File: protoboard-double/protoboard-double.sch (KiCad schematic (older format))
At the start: 23 parts, among them J1 MODULE_HEADER, J2 MODULE_HEADER, P1 CONN_01X22, P10 CONN_01X22, P11 CONN_01X22, P12 CONN_01X22, P13 CONN_01X22, P14 CONN_01X22, P15 CONN_01X22, P16 CONN_01X22, P17 CONN_01X22, P18 CONN_01X22, P19 CONN_01X22, P2 CONN_01X22, P3 CONN_01X22, P4 CONN_01X22, P5 CONN_01X22, P6 CONN_01X22, P7 CONN_01X22, P8 CONN_01X22, P9 CONN_01X22

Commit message: doublewide ready for production
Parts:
- SILK1: footprint parts:TESSEL-HEXAGON-LOGO -> parts:TESSEL-HEXAGON-LOGO-BACK
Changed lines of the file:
@@
 F 0 "SILK1" H 4750 1950 60  0000 C CNN
 F 1 "logo" H 4750 1850 60  0000 C CNN
-F 2 "parts:TESSEL-HEXAGON-LOGO" H 4750 1900 60  0001 C CNN
+F 2 "parts:TESSEL-HEXAGON-LOGO-BACK" H 4750 1900 60  0001 C CNN
 F 3 "" H 4750 1900 60  0000 C CNN
 	1    4750 1900

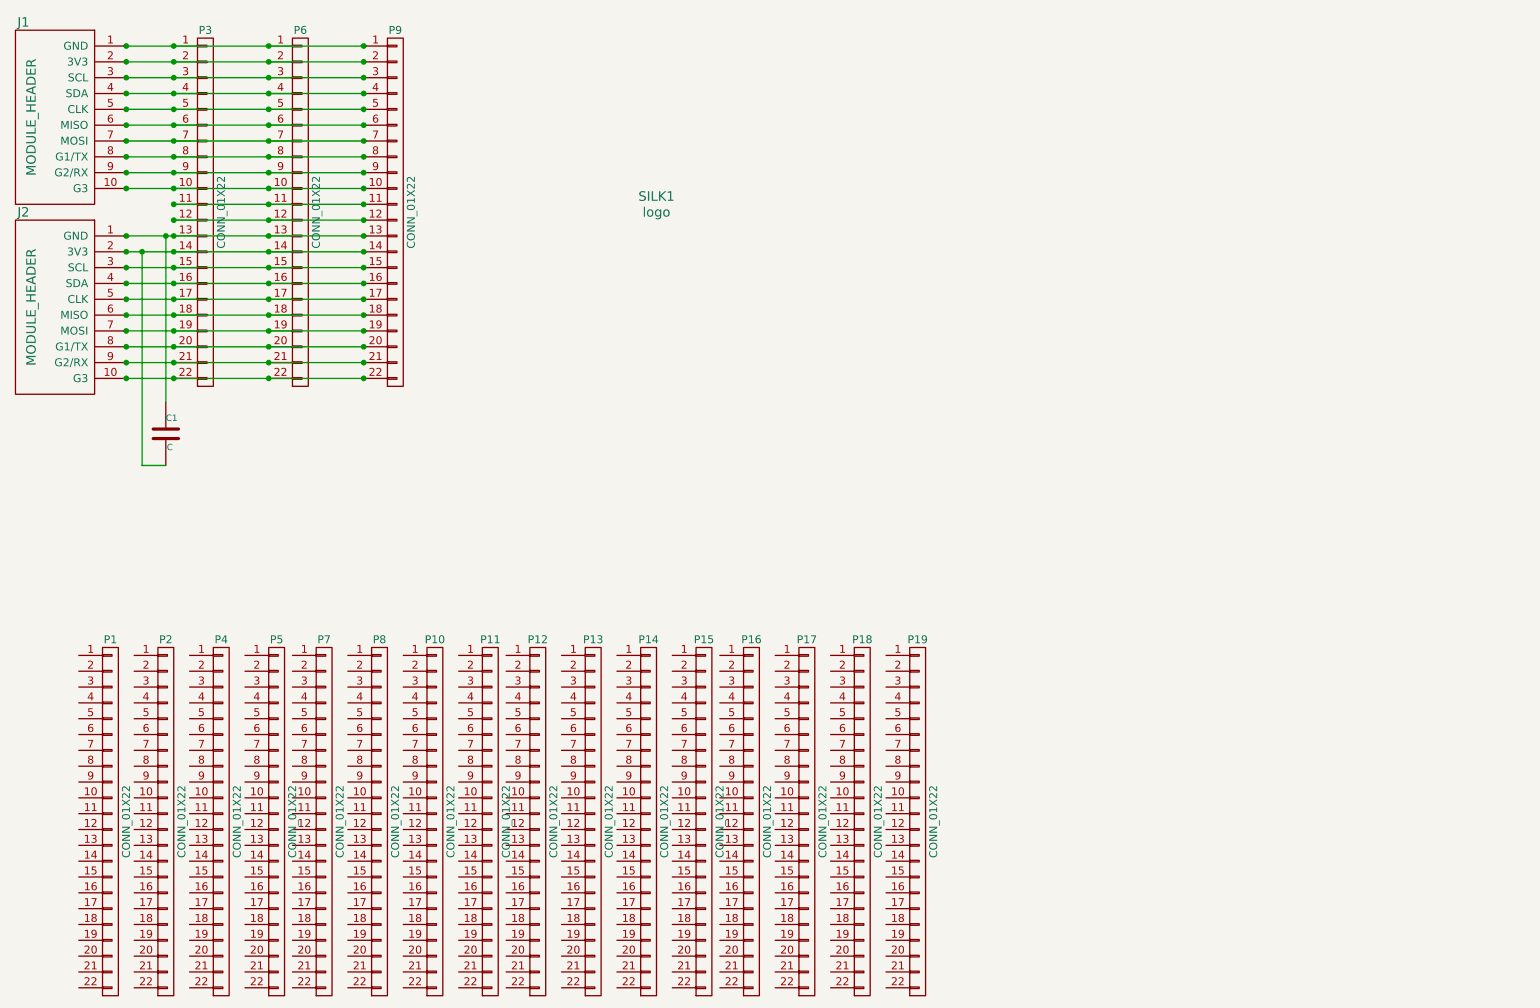
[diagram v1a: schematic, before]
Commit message: feedback incorporated for doublewide. all aboard the PCB ship!
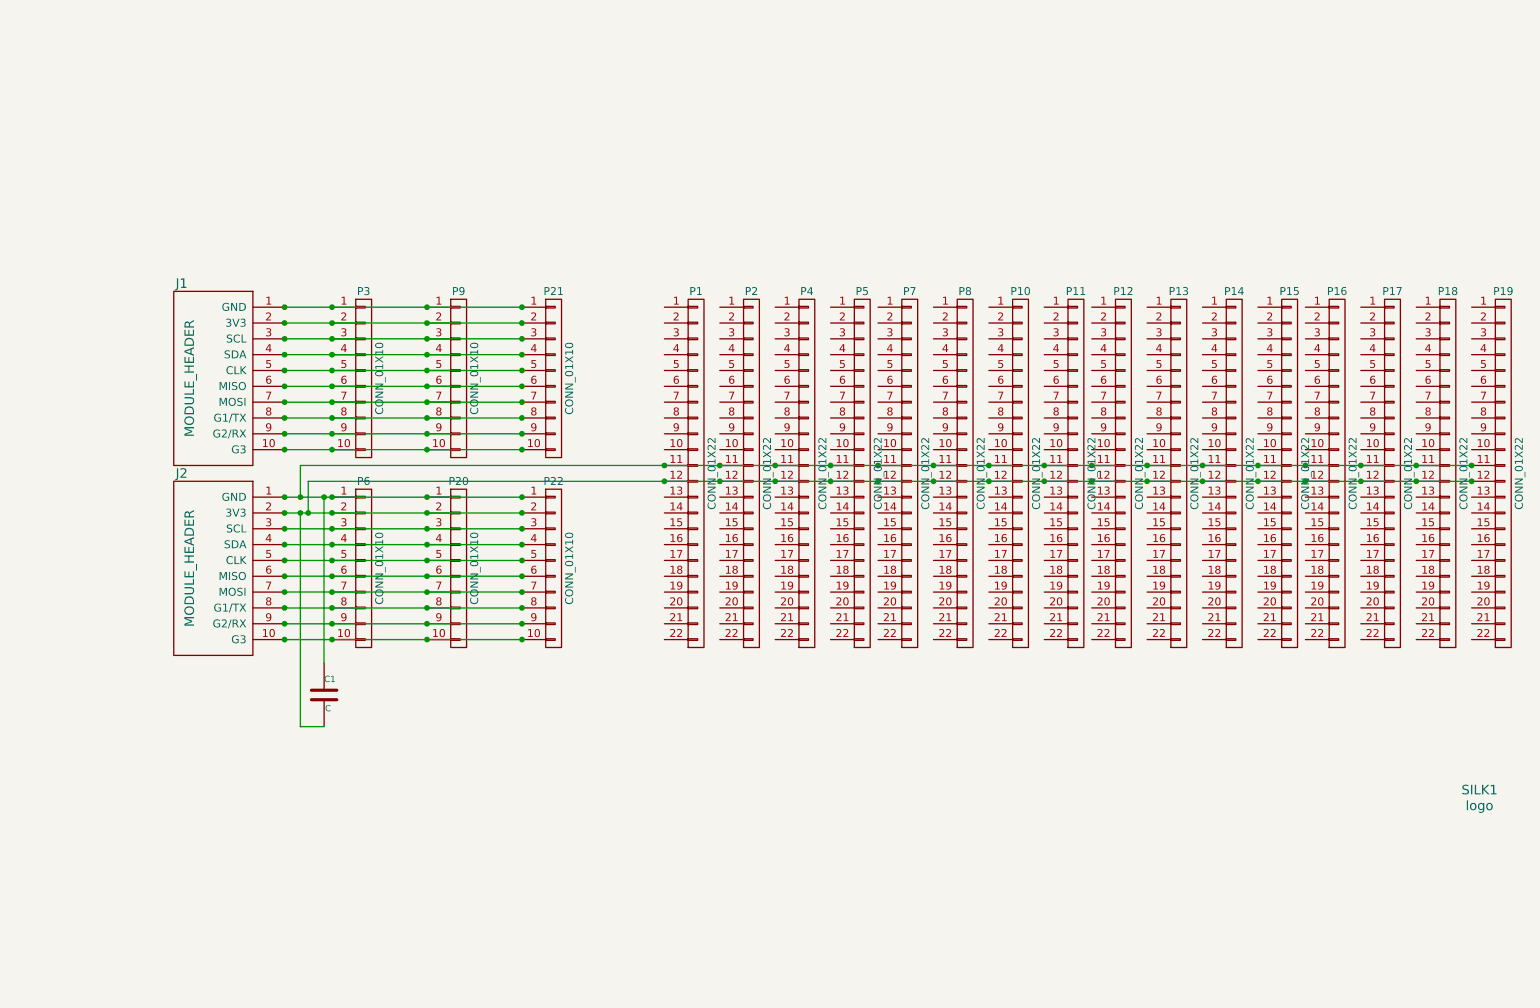
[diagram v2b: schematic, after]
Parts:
- removed P3, P6, P9: CONN_01X22, parts:1x22, symbol CONN_01X22
- added P20, P21, P22, P3, P6, P9: CONN_01X10, parts:1x10_BIG, symbol CONN_01X10
- J1, J2: footprint parts:MODULE_HEADER_MODULE -> parts:MODULE_HEADER_MODULE_BIG
- P1, P10, P11, P12, P13, P14, P15, P16, P17, P18, P19, P2, P4, P5, P7, P8: footprint parts:1x22 -> parts:1x22_BIG
- SILK1: footprint parts:TESSEL-HEXAGON-LOGO-BACK -> parts:TESSEL-HEXAGON-LOGO-BACK-BIG
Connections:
- net at J1.1 (GND): now also P21.1 (P1), P3.1 (P1), P9.1 (P1)
- net at J1.10 (G3): now also P21.10 (P10), P3.10 (P10), P9.10 (P10)
- net at J1.2 (3V3): now also P21.2 (P2), P3.2 (P2), P9.2 (P2)
- net at J1.3 (SCL): now also P21.3 (P3), P3.3 (P3), P9.3 (P3)
- net at J1.4 (SDA): now also P21.4 (P4), P3.4 (P4), P9.4 (P4)
- net at J1.5 (CLK): now also P21.5 (P5), P3.5 (P5), P9.5 (P5)
- net at J1.6 (MISO): now also P21.6 (P6), P3.6 (P6), P9.6 (P6)
- net at J1.7 (MOSI): now also P21.7 (P7), P3.7 (P7), P9.7 (P7)
- net at J1.8 (G1/TX): now also P21.8 (P8), P3.8 (P8), P9.8 (P8)
- net at J1.9 (G2/RX): now also P21.9 (P9), P3.9 (P9), P9.9 (P9)
- net at C1.1, J2.1 (GND): now also P1.11 (P11), P10.11 (P11), P11.11 (P11), P12.11 (P11), P13.11 (P11), P14.11 (P11), P15.11 (P11), P16.11 (P11), P17.11 (P11), P18.11 (P11), P19.11 (P11), P2.11 (P11), P4.11 (P11), P5.11 (P11), P7.11 (P11), P8.11 (P11), P20.1 (P1), P22.1 (P1), P6.1 (P1)
- net at J2.10 (G3): now also P20.10 (P10), P22.10 (P10), P6.10 (P10)
- net at C1.2, J2.2 (3V3): now also P1.12 (P12), P10.12 (P12), P11.12 (P12), P12.12 (P12), P13.12 (P12), P14.12 (P12), P15.12 (P12), P16.12 (P12), P17.12 (P12), P18.12 (P12), P19.12 (P12), P2.12 (P12), P4.12 (P12), P5.12 (P12), P7.12 (P12), P8.12 (P12), P20.2 (P2), P22.2 (P2), P6.2 (P2)
- net at J2.3 (SCL): now also P20.3 (P3), P22.3 (P3), P6.3 (P3)
- net at J2.4 (SDA): now also P20.4 (P4), P22.4 (P4), P6.4 (P4)
- net at J2.5 (CLK): now also P20.5 (P5), P22.5 (P5), P6.5 (P5)
- net at J2.6 (MISO): now also P20.6 (P6), P22.6 (P6), P6.6 (P6)
- net at J2.7 (MOSI): now also P20.7 (P7), P22.7 (P7), P6.7 (P7)
- net at J2.8 (G1/TX): now also P20.8 (P8), P22.8 (P8), P6.8 (P8)
- net at J2.9 (G2/RX): now also P20.9 (P9), P22.9 (P9), P6.9 (P9)
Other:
- moved on the sheet: C1, J1, J2, P1, P10, P11, P12, P13, P14, P15, P16, P17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
